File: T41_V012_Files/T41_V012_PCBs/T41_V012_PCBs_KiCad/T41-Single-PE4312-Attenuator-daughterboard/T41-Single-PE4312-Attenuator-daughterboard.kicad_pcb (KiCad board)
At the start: 2 copper layers, 14.6 x 17 mm, 8 parts, among them J1 Conn 1, J2 Conn 2, U1 PE4312

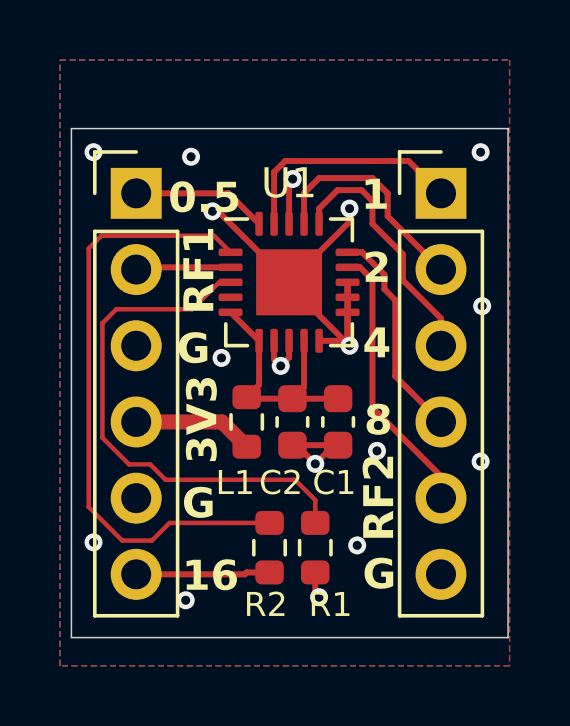
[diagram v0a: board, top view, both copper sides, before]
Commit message: Update
Update
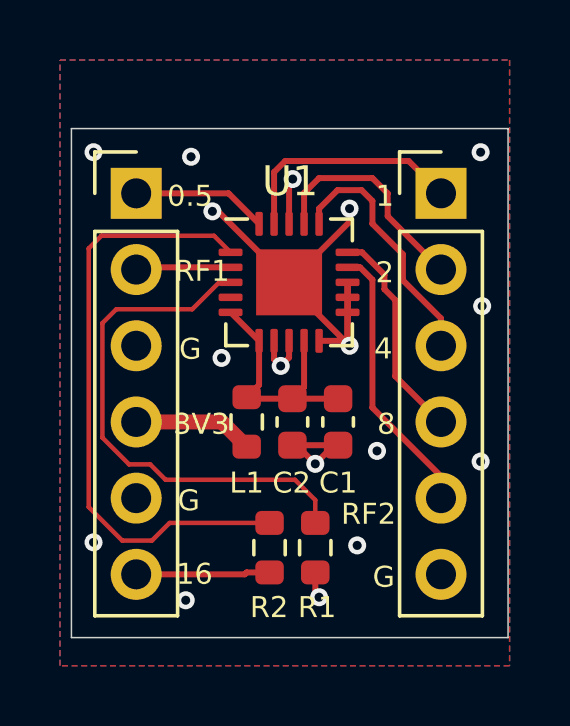
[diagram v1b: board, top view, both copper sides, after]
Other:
- board text added: "RFIN"
- board text added: "RFOUT"
- board text added: "T41 Attenuator Brd V2 06JUL26"
- board text removed: "RF"
- board text removed: "T41 Att. Brd V1 27DEC25"
